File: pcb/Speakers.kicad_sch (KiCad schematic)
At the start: 34 parts, among them U4 ADA4891, U7 ADA4891

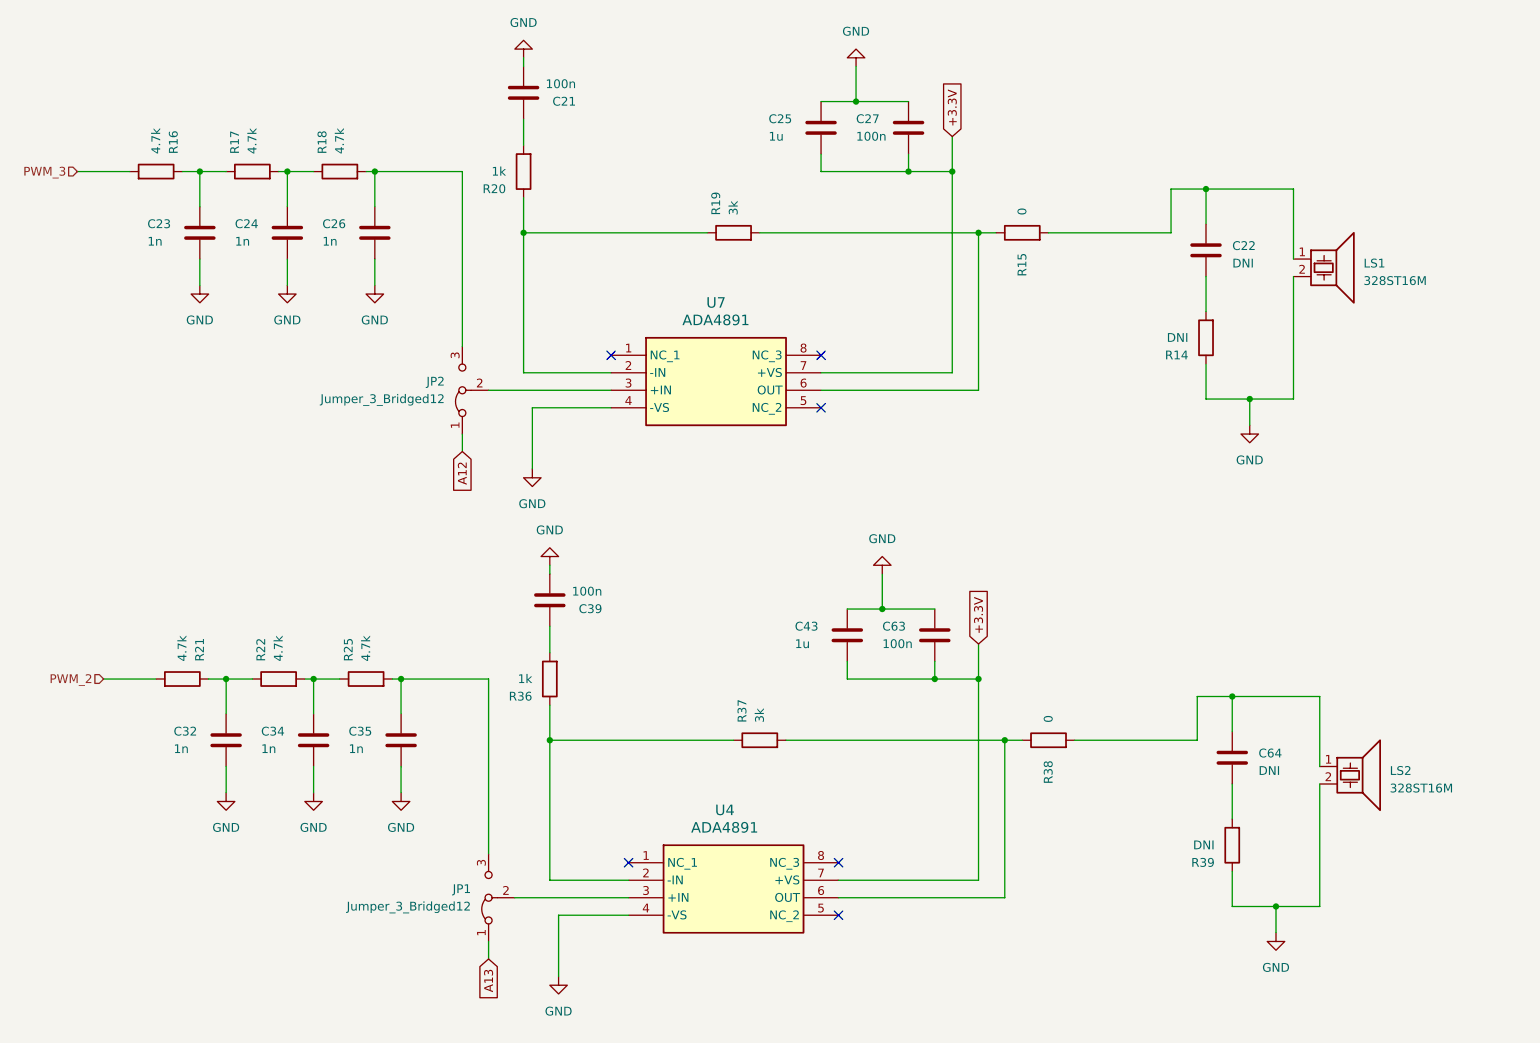
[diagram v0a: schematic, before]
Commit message: Polishin pt1
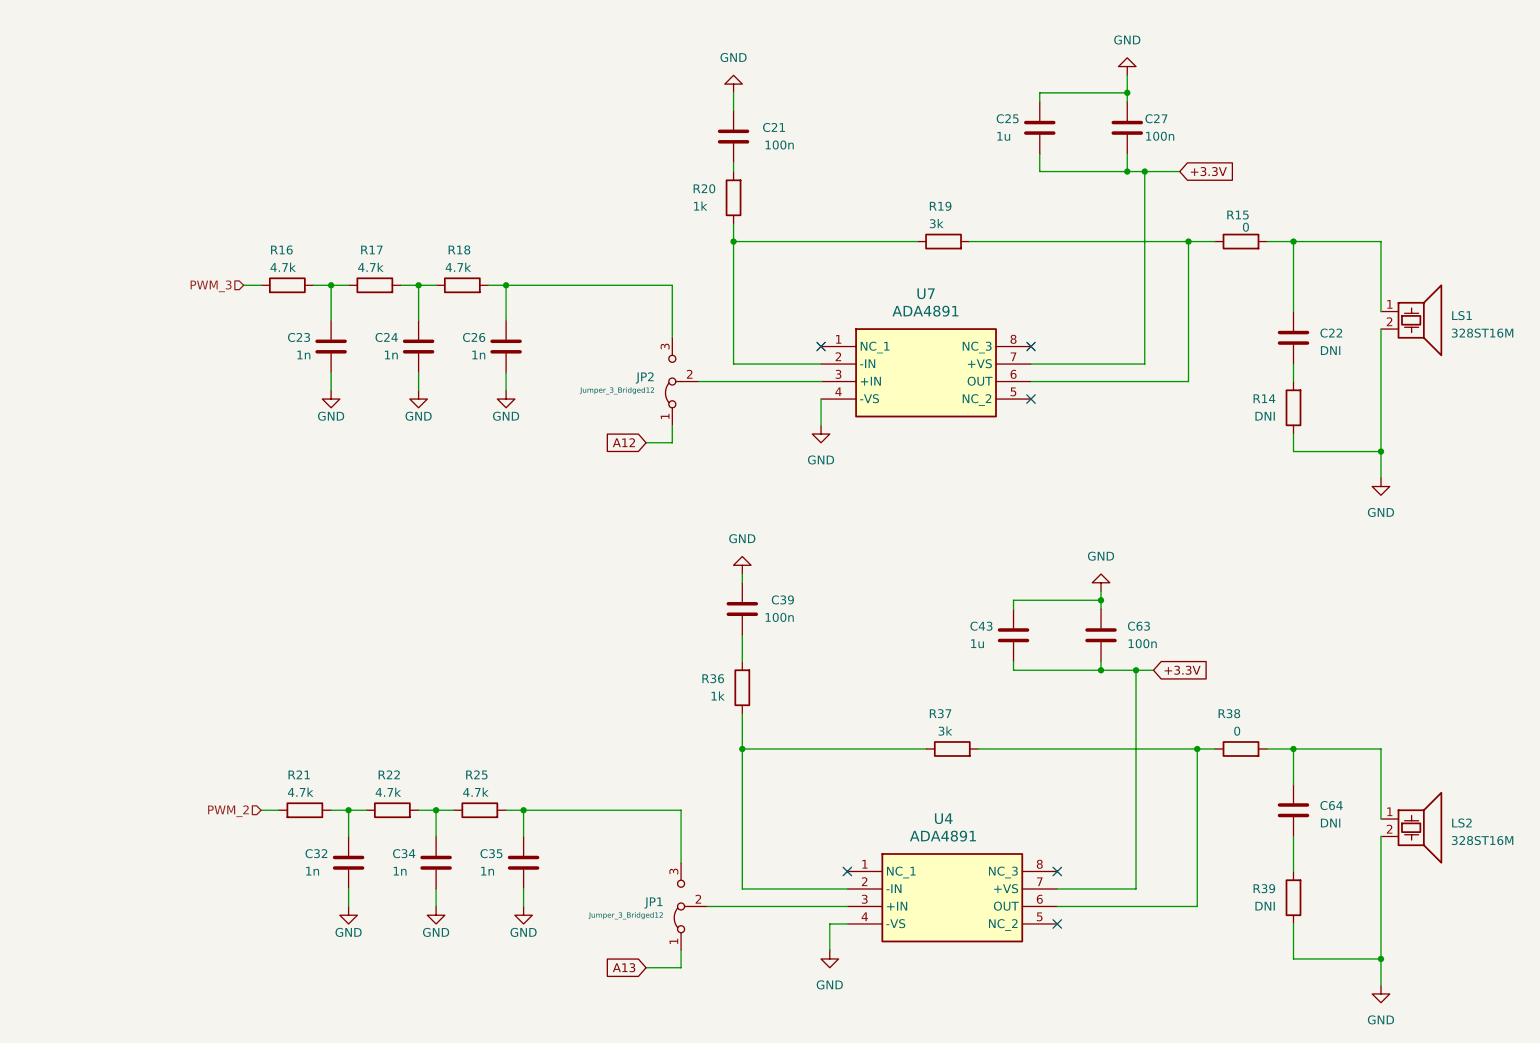
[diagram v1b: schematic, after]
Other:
- company: (none) -> Infineon Technologies
- title: (none) -> SensEdu 0.7
- moved on the sheet: C21, C22, C23, C24, C25, C26, C27, C32, C34, C35, C39, C43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
